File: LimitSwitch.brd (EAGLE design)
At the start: 7 x 22.2 mm, 3 parts, among them X1 53048-02

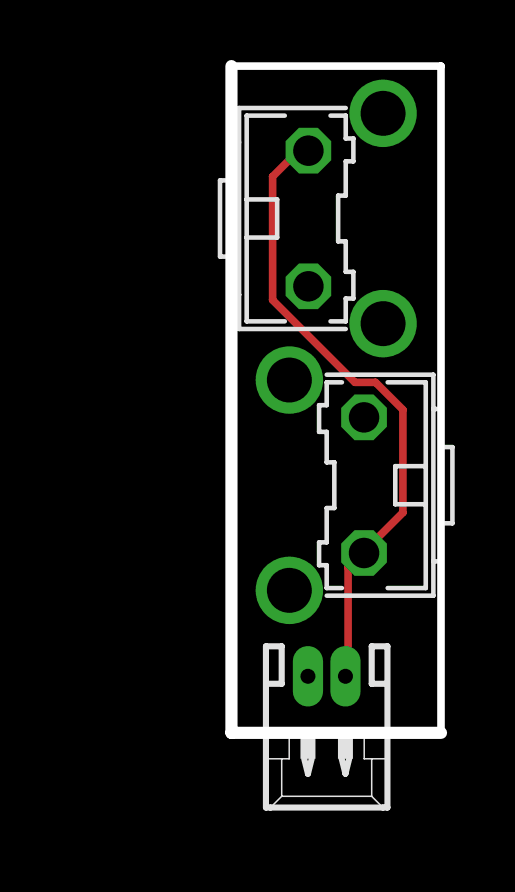
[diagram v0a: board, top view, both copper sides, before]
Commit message: sent off an order
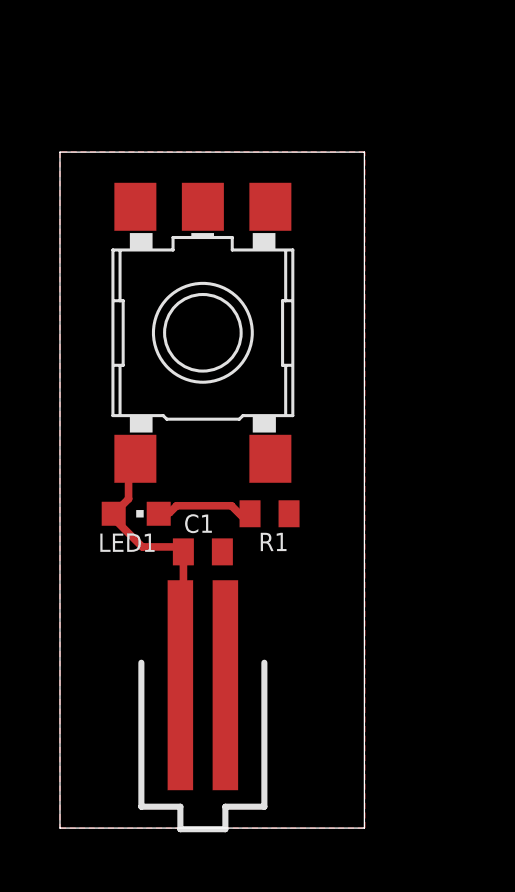
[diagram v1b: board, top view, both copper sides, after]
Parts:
- removed INSIDE, OUTSIDE: (no value), switch-omron:B3F-31XX
- removed X1: 53048-02, con-molex:53048-02
- added C1: GRM1555C1H471FA01D, resistor:C0402
- added LED1: LG Q396-PS-35, led:CHIPLED_0603
- added R1: ERJ-2RKF1004X, resistor:R0402
- added S2: SKHMPSE010, switch:SKHMPXE010
- added X2: 87438-02, con-molex:87438-02
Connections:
- new net N$1: LED1.C, R1.2
- net +: now also C1.1, LED1.A, S2.1, X2.1; no longer INSIDE.2, OUTSIDE.2, X1.1
- net GND: now also C1.2, R1.1, S2.3, S2.5, X2.2; no longer INSIDE.1, OUTSIDE.1, X1.2
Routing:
- net GND: track 21.3 -> 0.00 mm
- net +: track 0.00 -> 9.57 mm
- net N$1: track 0.00 -> 3.42 mm
- added copper zone on layer 1, net GND
- removed copper zone on layer 1, net +
- removed copper zone on layer 16, net GND
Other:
- board size 7 x 22.2 mm -> 10.1 x 22.5 mm
